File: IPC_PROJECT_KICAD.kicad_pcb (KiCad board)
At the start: 2 copper layers, 125.2 x 70 mm, 142 parts, among them IC1 ESP32-C3-MINI-1-N4-A, J1 JUMPER, J2 JFP1, J3 691322310010, J4 JUSB1, Q1 MMBT3904, Q2 MMBT3904, Q3 MMBT3904, Q4 MMBT3904, Q5 MMBT3904, Q6 MMBT3904, U1 LM35-LP, U10 PC817, U11 PCN-105D3MHZ, U12 PC817, U13 PCN-105D3MHZ, U14 PC817, U15 PC817, U16 PC817, U17 PC817, U18 PC817, U19 USBLC6-2SC6, U2 TPS26602PWP, U20 TPS54360DDA, U21 AP7361C-33E, U3 PCN-105D3MHZ, U4 PCN-105D3MHZ, U5 PC817, U6 PC817, U7 PCN-105D3MHZ, U8 PCN-105D3MHZ, U9 PC817

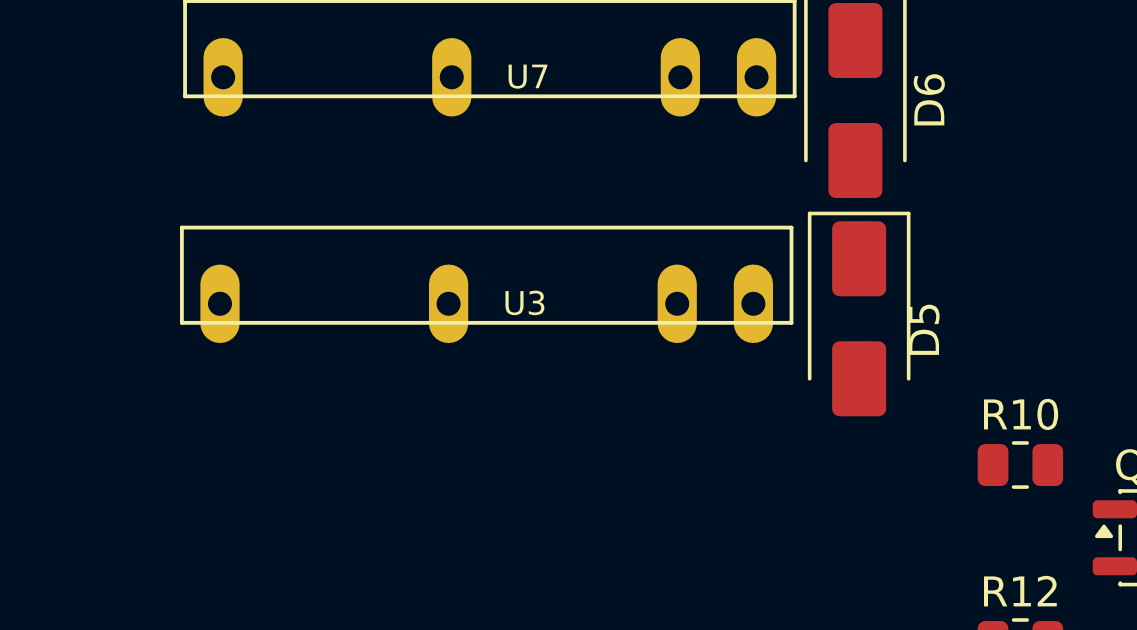
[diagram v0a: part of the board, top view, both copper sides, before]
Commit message: Add files via upload
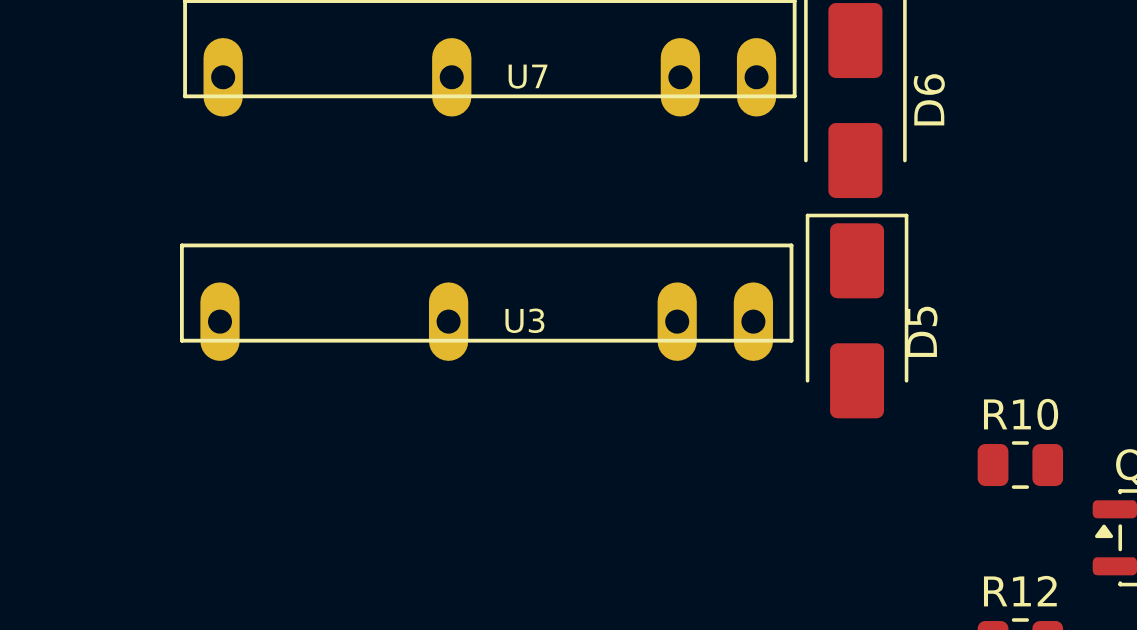
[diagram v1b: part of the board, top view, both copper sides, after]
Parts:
- moved U3 0.59 mm to (108.1, 103.6)
- moved D5 0.10 mm to (119.1, 103.6)
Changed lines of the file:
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@@
 	(footprint "PCN-105D3MHZ:PCN-105D3MHZ"
 		(layer "F.Cu")
-		(at 108.055 103.025 180)
+		(at 108.055 103.62 180)
 		(descr "Single contact 5V relay")
 		(property "Reference" "U3"
@@
 	(footprint "Diode_SMD:D_SMA"
 		(layer "F.Cu")
-		(at 119.2 103.525 -90)
+		(at 119.13 103.5925 -90)
 		(descr "Diode SMA (DO-214AC)")
 		(tags "Diode SMA (DO-214AC)")
